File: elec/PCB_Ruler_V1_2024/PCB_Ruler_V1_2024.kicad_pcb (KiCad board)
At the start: 2 copper layers, 51 parts, among them J1 USB-C, J2 S2B-XH-A-1LFSN, SW1 CS1213AGF260, SW2 CS1213AGF260, SW3 CS1213AGF260, SW4 CS1213AGF260, SW5 CS1213AGF260, SW6 CS1213AGF260, SW7 CS1213AGF260, U1 ESP32-C3-WROOM-02-H4, U2 MCP73831T-2ACI_OT, U3 TLV75533PDBV, U4 TCA9534PWR, U5 VL53L4CXV0DH/1

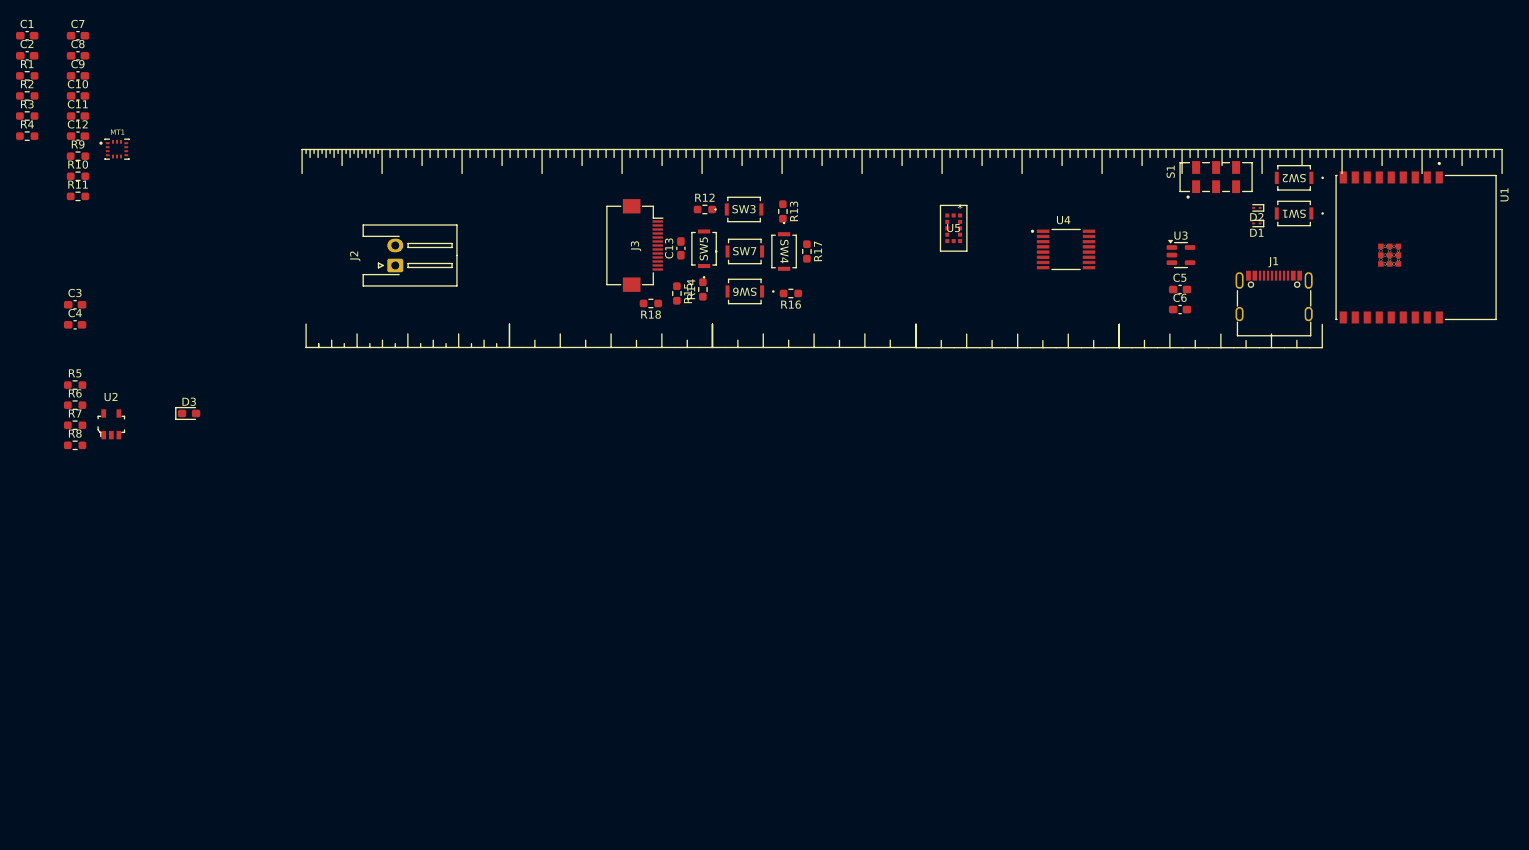
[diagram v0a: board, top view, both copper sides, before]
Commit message: idk
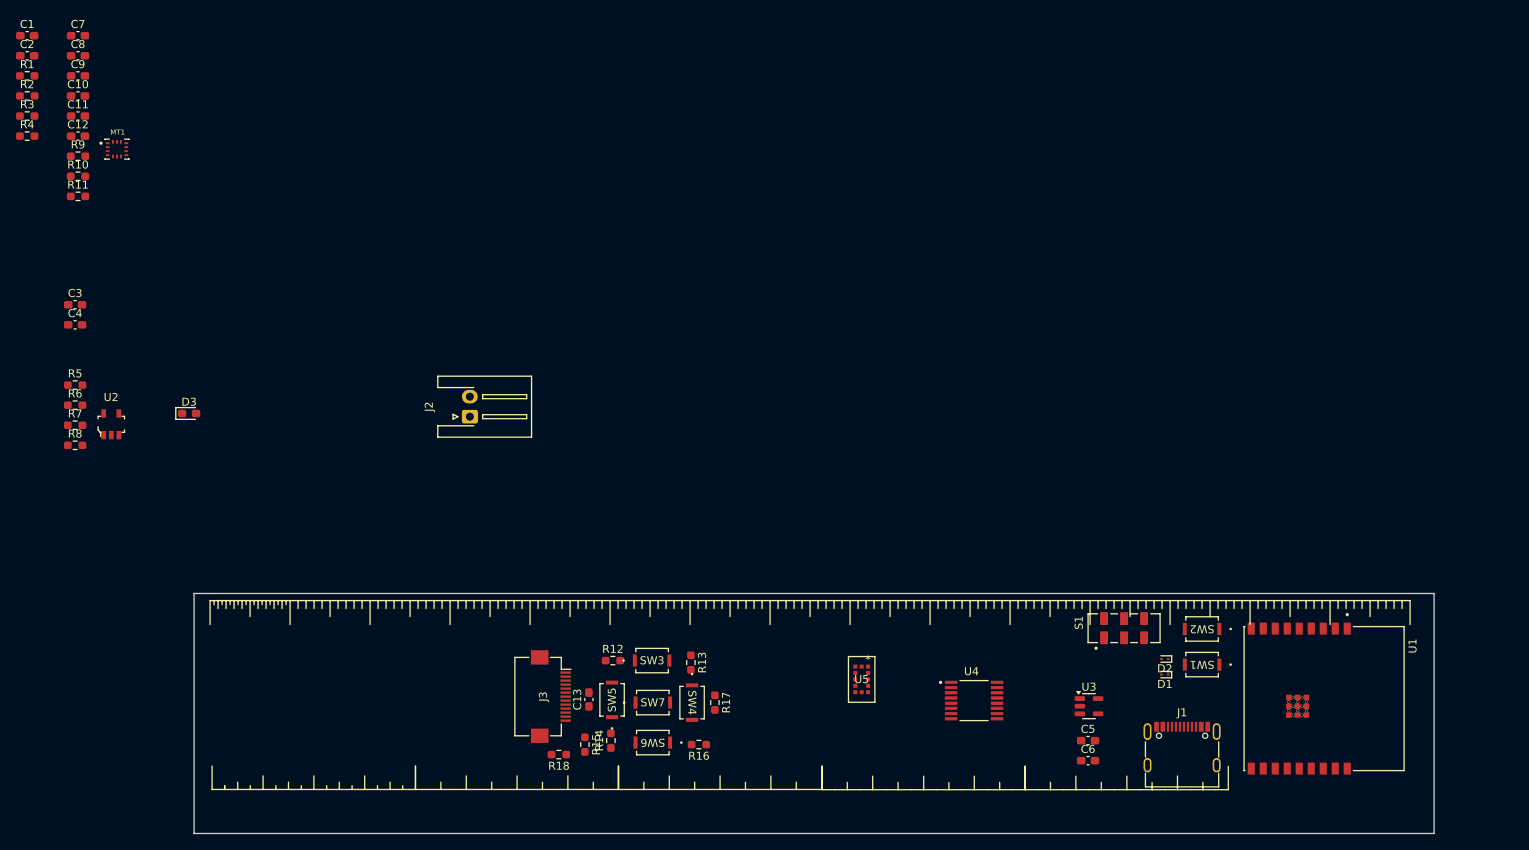
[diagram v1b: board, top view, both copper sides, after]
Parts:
- moved D2 57.6 mm to (219.8, 130.7)
- moved U5 57.6 mm to (182.0, 133.2)
- moved C13 57.6 mm to (147.9, 135.8)
- moved C6 57.6 mm to (210.2, 143.4)
- moved D1 57.6 mm to (219.8, 132.6)
- moved S1 57.6 mm to (214.8, 126.8)
- moved SW2 57.6 mm to (224.5, 126.9)
- moved SW5 57.6 mm to (150.8, 135.8)
- moved U3 57.6 mm to (210.4, 136.6)
- moved C5 57.6 mm to (210.2, 140.9)
- moved J1 57.6 mm to (222.0, 142.9)
- moved J3 57.6 mm to (143.1, 135.4)
- moved R12 57.6 mm to (150.9, 130.9)
- moved R13 57.6 mm to (160.6, 131.1)
- moved R14 57.6 mm to (150.6, 140.9)
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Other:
- board outline added: 155 x 30 mm
